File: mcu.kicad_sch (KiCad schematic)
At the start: 26 parts, among them SW400 TL2243, U400 STM32F750V8Tx, X300 Q13FC1350000400, X400 X322512MSB4SI

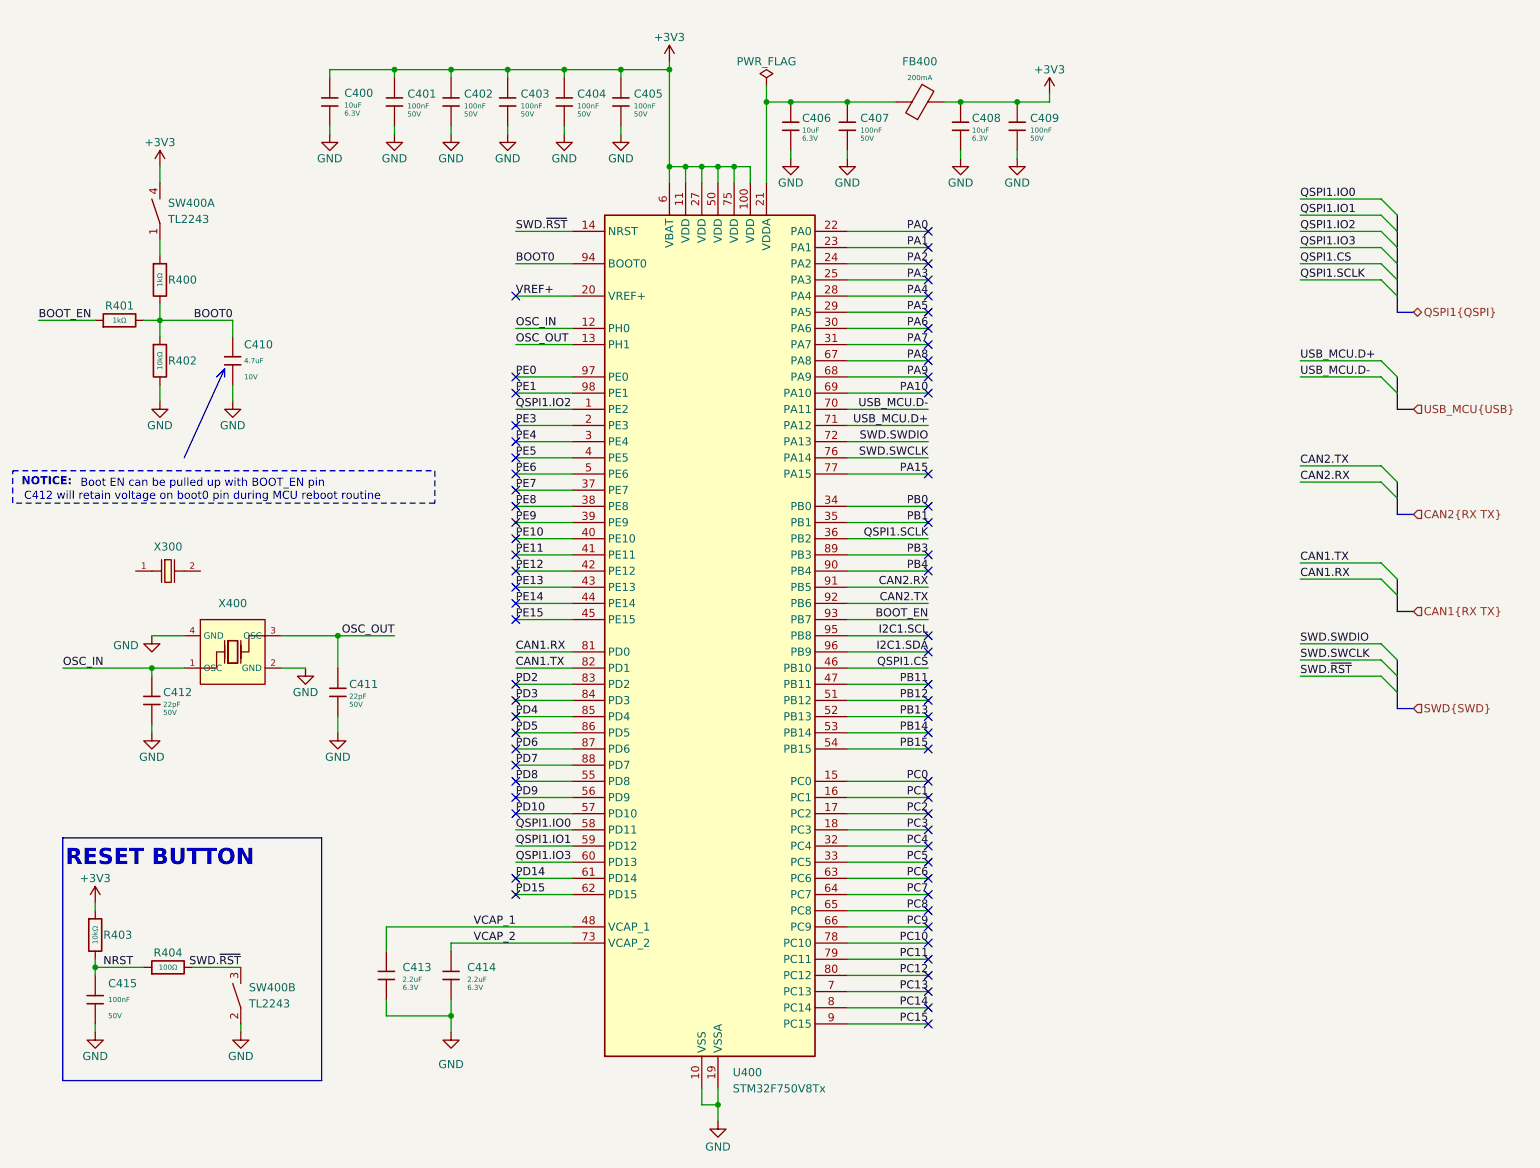
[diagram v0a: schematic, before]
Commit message: [#2] Fix MCU model, draft QSPI connection
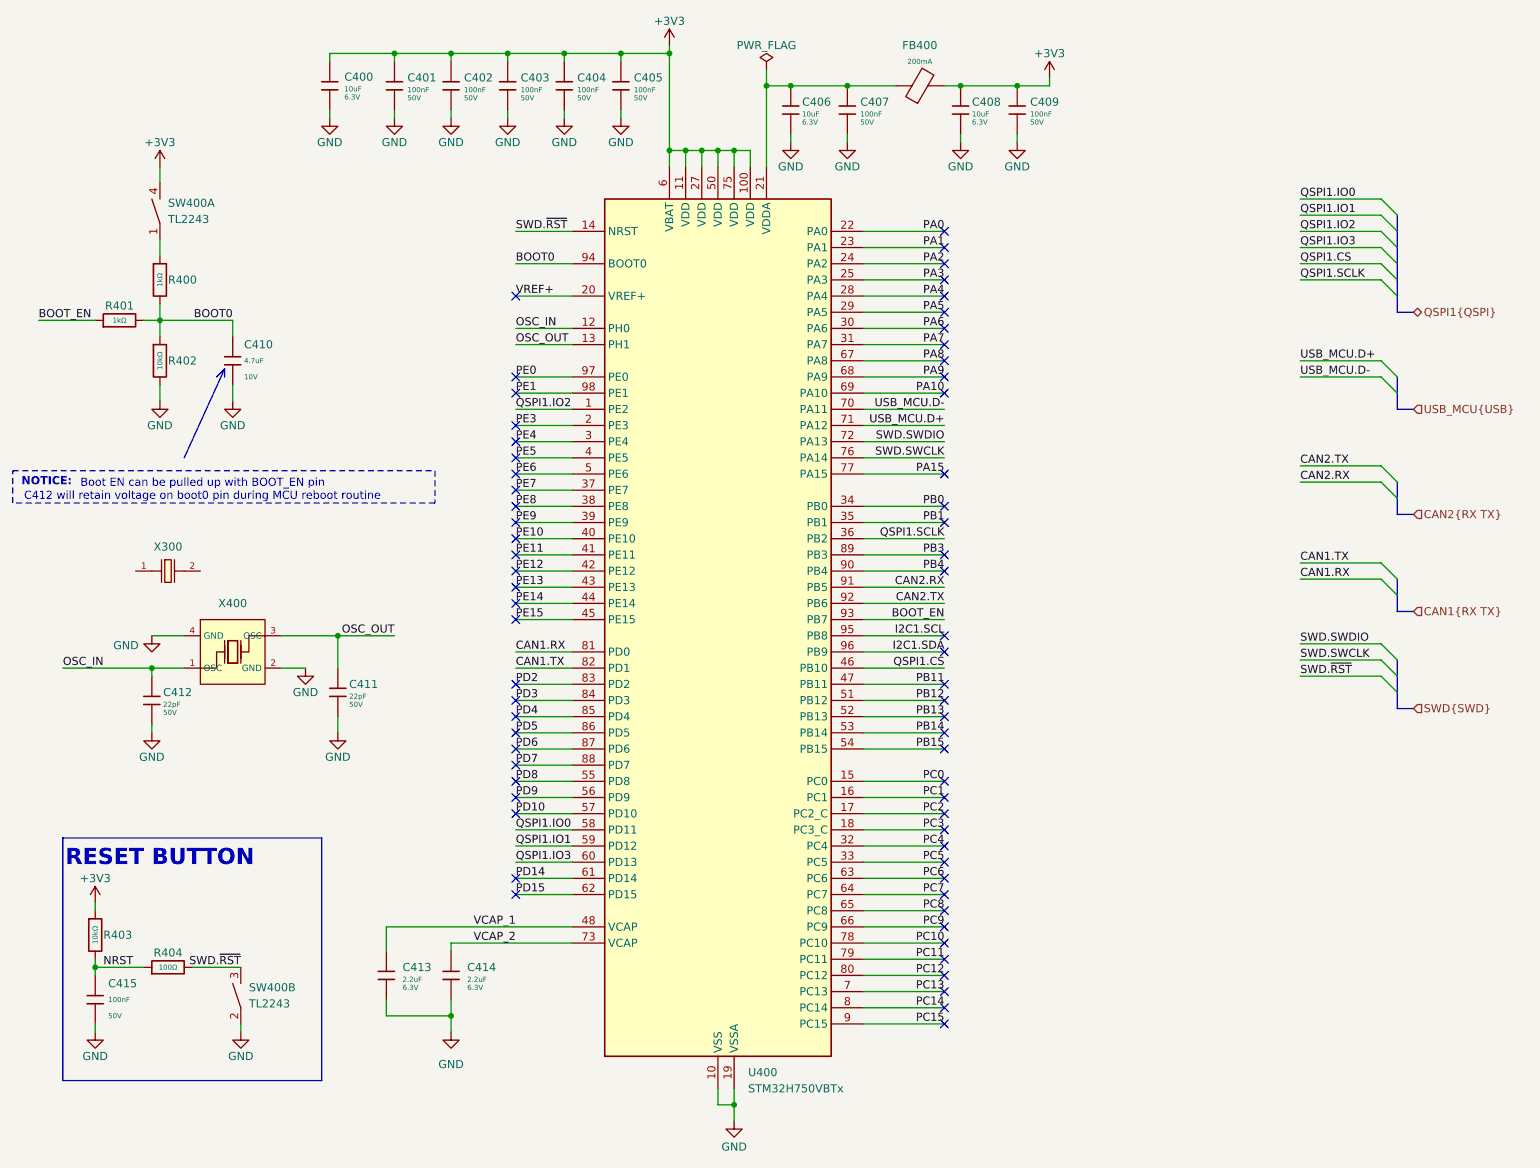
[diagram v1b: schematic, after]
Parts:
- removed U400: STM32F750V8Tx, Package_QFP:LQFP-100_14x14mm_P0.5mm, symbol MCU_ST_STM32F7:STM32F750V8Tx
- added U400: STM32H750VBTx, Package_QFP:LQFP-100_14x14mm_P0.5mm, symbol MCU_ST_STM32H7:STM32H750VBTx
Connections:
- net +3V3: now also U400.100 (VDD), U400.11 (VDD), U400.27 (VDD), U400.50 (VDD), U400.6 (VBAT), U400.75 (VDD)
- net BOOT0: now also U400.94 (BOOT0)
- net BOOT_EN: now also U400.93 (PB7)
- net CAN1.RX: now also U400.81 (PD0)
- net CAN1.TX: now also U400.82 (PD1)
- net CAN2.RX: now also U400.91 (PB5)
- net CAN2.TX: now also U400.92 (PB6)
- net GND: now also U400.10 (VSS), U400.19 (VSSA), U400.26 (VSS), U400.49 (VSS), U400.74 (VSS), U400.99 (VSS)
- net I2C1.SCL: now also U400.95 (PB8)
- net I2C1.SDA: now also U400.96 (PB9)
- net OSC_IN: now also U400.12 (PH0)
- net OSC_OUT: now also U400.13 (PH1)
- net PA0: now also U400.22 (PA0)
- net PA1: now also U400.23 (PA1)
- net PA10: now also U400.69 (PA10)
- net PA15: now also U400.77 (PA15)
- net PA2: now also U400.24 (PA2)
- net PA3: now also U400.25 (PA3)
- net PA4: now also U400.28 (PA4)
- net PA5: now also U400.29 (PA5)
- net PA6: now also U400.30 (PA6)
- net PA7: now also U400.31 (PA7)
- net PA8: now also U400.67 (PA8)
- net PA9: now also U400.68 (PA9)
- net PB0: now also U400.34 (PB0)
- net PB1: now also U400.35 (PB1)
- net PB11: now also U400.47 (PB11)
- net PB12: now also U400.51 (PB12)
- net PB13: now also U400.52 (PB13)
- net PB14: now also U400.53 (PB14)
- net PB15: now also U400.54 (PB15)
- net PB3: now also U400.89 (PB3)
- net PB4: now also U400.90 (PB4)
- net PC0: now also U400.15 (PC0)
- net PC1: now also U400.16 (PC1)
- net PC10: now also U400.78 (PC10)
- net PC11: now also U400.79 (PC11)
- net PC12: now also U400.80 (PC12)
- net PC13: now also U400.7 (PC13)
- net PC14: now also U400.8 (PC14)
- net PC15: now also U400.9 (PC15)
- net PC2: now also U400.17 (PC2_C)
- net PC3: now also U400.18 (PC3_C)
- net PC4: now also U400.32 (PC4)
- net PC5: now also U400.33 (PC5)
- net PC6: now also U400.63 (PC6)
- net PC7: now also U400.64 (PC7)
- net PC8: now also U400.65 (PC8)
- net PC9: now also U400.66 (PC9)
- net PD10: now also U400.57 (PD10)
- net PD14: now also U400.61 (PD14)
- net PD15: now also U400.62 (PD15)
- net PD2: now also U400.83 (PD2)
- net PD3: now also U400.84 (PD3)
- net PD4: now also U400.85 (PD4)
- net PD5: now also U400.86 (PD5)
- net PD6: now also U400.87 (PD6)
- net PD7: now also U400.88 (PD7)
- net PD8: now also U400.55 (PD8)
- net PD9: now also U400.56 (PD9)
- net PE0: now also U400.97 (PE0)
- net PE1: now also U400.98 (PE1)
- net PE10: now also U400.40 (PE10)
- net PE11: now also U400.41 (PE11)
- net PE12: now also U400.42 (PE12)
- net PE13: now also U400.43 (PE13)
- net PE14: now also U400.44 (PE14)
- net PE15: now also U400.45 (PE15)
- net PE3: now also U400.2 (PE3)
- net PE4: now also U400.3 (PE4)
- net PE5: now also U400.4 (PE5)
- net PE6: now also U400.5 (PE6)
- net PE7: now also U400.37 (PE7)
- net PE8: now also U400.38 (PE8)
- net PE9: now also U400.39 (PE9)
- net QSPI1.CS: now also U400.46 (PB10)
- net QSPI1.IO0: now also U400.58 (PD11)
- net QSPI1.IO1: now also U400.59 (PD12)
- net QSPI1.IO2: now also U400.1 (PE2)
- net QSPI1.IO3: now also U400.60 (PD13)
- net QSPI1.SCLK: now also U400.36 (PB2)
- net SWD.SWCLK: now also U400.76 (PA14)
- net SWD.SWDIO: now also U400.72 (PA13)
- net SWD.~{RST}: now also U400.14 (NRST)
- net USB_MCU.D+: now also U400.71 (PA12)
- net USB_MCU.D-: now also U400.70 (PA11)
- net VCAP_1: now also U400.48 (VCAP)
- net VCAP_2: now also U400.73 (VCAP)
- net VREF+: now also U400.20 (VREF+)
- net at C406.1, C407.1, FB400.1: now also U400.21 (VDDA)
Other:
- moved on the sheet: C400, C401, C402, C403, C404, C405, C406, C407, C408, C409, FB400
